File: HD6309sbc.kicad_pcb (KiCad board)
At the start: 4 copper layers, 99.8 x 99.8 mm, 86 parts, among them J1 Conn_01x02_Male, J2 Conn_02x30_Odd_Even, J3 Conn_01x02_Male, J4 Conn_01x07_Socket, J5 Conn_01x07_Socket, J6 PD0, J7 PD1, SW1 SW_Push, U1 HD63C09, U12 74HCT138, U16 74HCT541, U19 74HCT30, U2 DS1813, U3 74AHC1G14, U4 74HCT138, U5 GAL16V8, U6 74HCT574, U7 74HCT574, U8 74HCT541

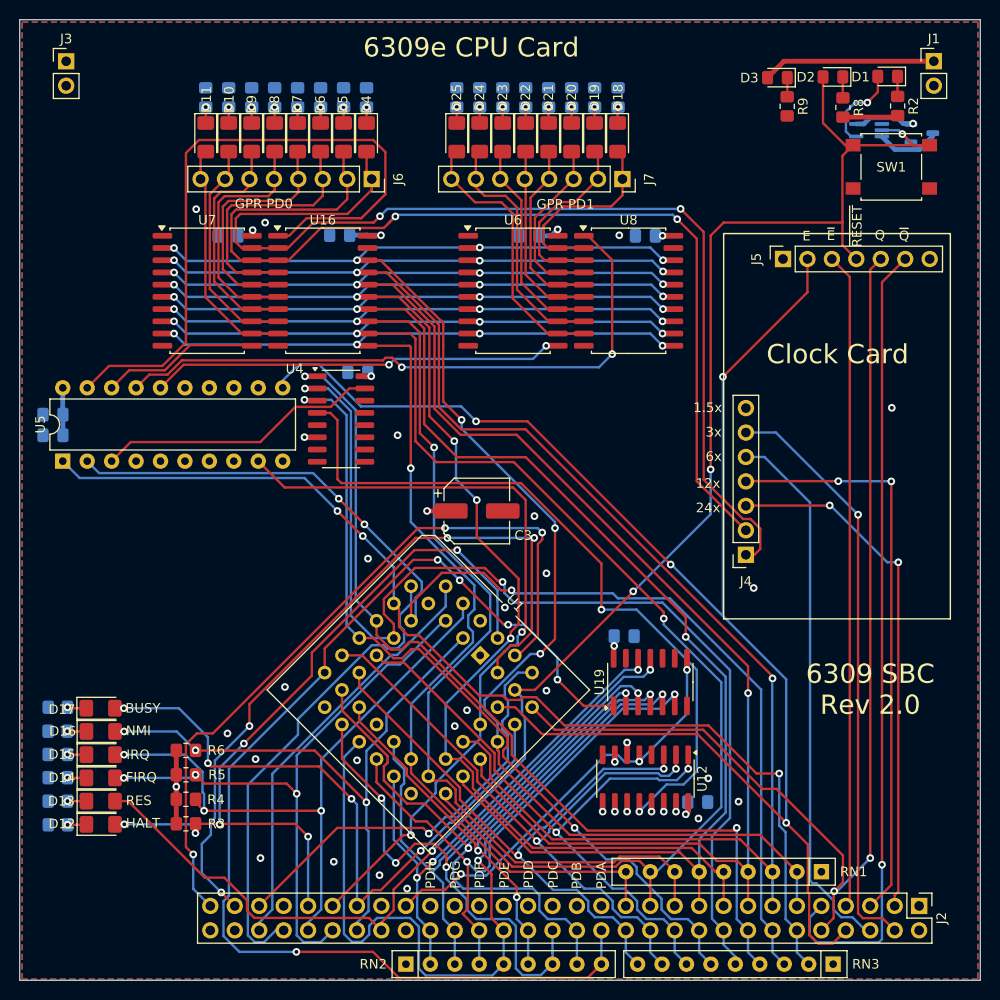
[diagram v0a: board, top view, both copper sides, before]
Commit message: update readme
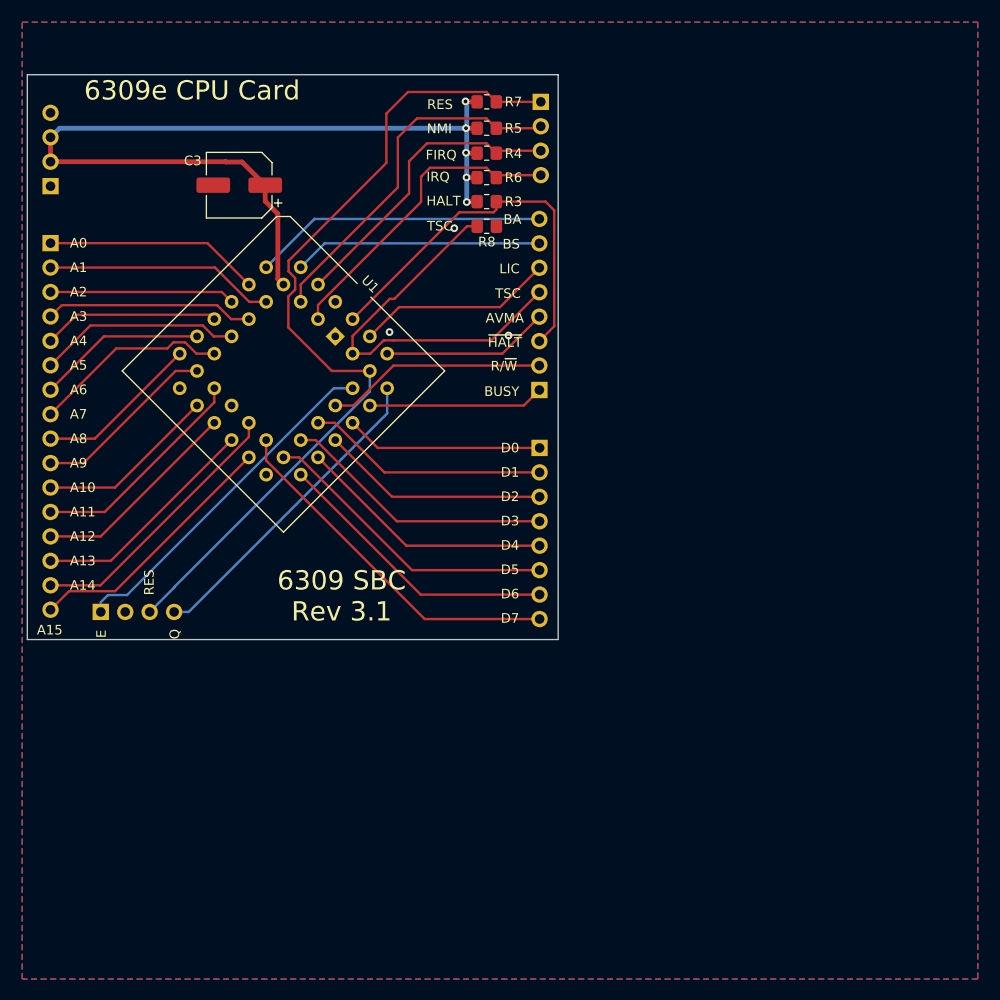
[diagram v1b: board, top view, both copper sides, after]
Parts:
- removed C1, C10, C2, C4, C5, C6, C7, C8, C9: 10uF, Capacitor_SMD:C_0805_2012Metric_Pad1.18x1.45mm_HandSolder
- removed D1: RED, LED_SMD:LED_0805_2012Metric_Pad1.15x1.40mm_HandSolder
- removed D10, D11, D12, D13, D14, D15, D16, D17, D18, D19, D20, D21, D22, D23, D24, D25, D4, D5, D6, D7, D8, D9: LED_Filled, LED_SMD:LED_1206_3216Metric_Pad1.42x1.75mm_HandSolder
- removed D2: YELLOW, LED_SMD:LED_0805_2012Metric_Pad1.15x1.40mm_HandSolder
- removed D3: GREEN, LED_SMD:LED_0805_2012Metric_Pad1.15x1.40mm_HandSolder
- removed J1, J3: Conn_01x02_Male, Connector_PinHeader_2.54mm:PinHeader_1x02_P2.54mm_Vertical
- removed R1, R10, R11, R12, R13, R14, R15, R16, R17, R18, R19, R20, R21, R22, R23, R24, R25, R26, R27, R28, R29: 470R, Resistor_SMD:R_0805_2012Metric_Pad1.20x1.40mm_HandSolder
- removed R2, R9: 330R, Resistor_SMD:R_0805_2012Metric_Pad1.20x1.40mm_HandSolder
- removed RN1, RN2, RN3: 4K7, Resistor_THT:R_Array_SIP9
- removed SW1: SW_Push, Button_Switch_SMD:SW_SPST_B3S-1000
- removed U12, U4: 74HCT138, Package_SO:SOIC-16_3.9x9.9mm_P1.27mm
- removed U16, U8: 74HCT541, Package_SO:SOIC-20W_7.5x12.8mm_P1.27mm
- removed U19: 74HCT30, Package_SO:SOIC-14_3.9x8.7mm_P1.27mm
- removed U2: DS1813, Package_TO_SOT_SMD:SOT-23-3
- removed U3: 74AHC1G14, Package_TO_SOT_SMD:SOT-353_SC-70-5_Handsoldering
- removed U5: GAL16V8, Package_DIP:DIP-20_W7.62mm
- removed U6, U7: 74HCT574, Package_SO:SOIC-20W_7.5x12.8mm_P1.27mm
- added J8: Interrupts, Connector_PinHeader_2.54mm:PinHeader_1x04_P2.54mm_Vertical, B.Cu at (79.6, 33.9)
- J2: value Conn_02x30_Odd_Even -> Address Bus; footprint Connector_PinHeader_2.54mm:PinHeader_2x30_P2.54mm_Vertical -> Connector_PinHeader_2.54mm:PinHeader_1x16_P2.54mm_Vertical; moved to B.Cu
- J4: value Conn_01x07_Socket -> Power; footprint Connector_PinSocket_2.54mm:PinSocket_1x07_P2.54mm_Vertical -> Connector_PinHeader_2.54mm:PinHeader_1x04_P2.54mm_Vertical; moved to B.Cu
- J5: value Conn_01x07_Socket -> quadrature; footprint Connector_PinSocket_2.54mm:PinSocket_1x07_P2.54mm_Vertical -> Connector_PinSocket_2.54mm:PinSocket_1x04_P2.54mm_Vertical; moved to B.Cu
- J6: value PD0 -> Data Bus; footprint Connector_PinSocket_2.54mm:PinSocket_1x08_P2.54mm_Vertical -> Connector_PinHeader_2.54mm:PinHeader_1x08_P2.54mm_Vertical; moved to B.Cu
- J7: value PD1 -> CPU Control; footprint Connector_PinSocket_2.54mm:PinSocket_1x08_P2.54mm_Vertical -> Connector_PinHeader_2.54mm:PinHeader_1x08_P2.54mm_Vertical; moved to B.Cu
- R7: value 470R -> 4.7k; moved to F.Cu
- R8: value 330R -> 4.7k
- moved J2 113.5 mm to (28.6, 48.6), turned to 180 degrees
- moved J4 81.8 mm to (28.6, 42.7), turned to 0 degrees
- moved J5 79.8 mm to (33.8, 86.9), turned to -90 degrees
- moved R5 74.1 mm to (73.9, 36.7)
- moved R4 74.1 mm to (73.9, 39.3)
- moved R3 71.8 mm to (73.9, 44.3)
- moved R6 67.2 mm to (73.9, 41.8)
- moved C3 41.9 mm to (48.2, 42.6), turned to 180 degrees
- moved R8 39.0 mm to (73.9, 46.9), turned to 0 degrees
- moved U1 36.4 mm to (58.2, 58.3)
- moved J6 32.9 mm to (79.4, 69.9), turned to 180 degrees
- moved J7 23.6 mm to (79.4, 63.9), turned to 0 degrees
- moved R7 14.9 mm to (73.9, 33.9), turned to 0 degrees
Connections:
- J2 pad 1: unconnected-(J2-Pin_1-Pad1) -> /A0
- J2 pad 10: Q -> /A9
- J2 pad 11: /D0 -> /A10
- J2 pad 12: /A0 -> /A11
- J2 pad 13: /D1 -> /A12
- J2 pad 14: /A1 -> /A13
- J2 pad 15: /D2 -> /A14
- J2 pad 16: /A2 -> /A15
- J2 pad 2: +5V -> /A1
- J2 pad 3: Clock24 -> /A2
- J2 pad 4: Clock3 -> /A3
- J2 pad 5: Clock12 -> /A4
- J2 pad 6: Clock6 -> /A5
- J2 pad 7: ~{E} -> /A6
- J2 pad 8: E -> /A7
- J2 pad 9: ~{Q} -> /A8
- J4 pad 1: /ClockCard/intD00 -> GND
- J4 pad 2: /ClockCard/intD01 -> +5V
- J4 pad 3: Clock24 -> +5V
- J4 pad 4: Clock12 -> GND
- J5 pad 1: GND -> E
- J5 pad 2: E -> unconnected-(J5-Pin_2-Pad2)
- J5 pad 3: ~{E} -> ~{RESET}
- J5 pad 4: ~{RESET} -> Q
- J6 pad 1: /ClockCard/intD00 -> /D0
- J6 pad 2: /ClockCard/intD01 -> /D1
- J6 pad 3: /ClockCard/intD02 -> /D2
- J6 pad 4: /ClockCard/intD03 -> /D3
- J6 pad 5: /ClockCard/intD04 -> /D4
- J6 pad 6: /ClockCard/intD05 -> /D5
- J6 pad 7: /ClockCard/intD06 -> /D6
- J6 pad 8: /ClockCard/intD07 -> /D7
- J7 pad 1: /intD10 -> BUSY
- J7 pad 2: /intD11 -> R/~{W}
- J7 pad 3: /intD12 -> ~{HALT}
- J7 pad 4: /intD13 -> AVMA
- J7 pad 5: /intD14 -> TSC
- J7 pad 6: /intD15 -> LIC
- J7 pad 7: /intD16 -> BS
- J7 pad 8: /intD17 -> BA
- R7 pad 1: Net-(D5-K) -> +5V
- R7 pad 2: GND -> ~{RESET}
- R8 pad 1: Net-(D2-K) -> TSC
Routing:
- net /D1: track 184.6 -> 25.2 mm, vias 5 -> 0
- net /D2: track 176.6 -> 23.7 mm, vias 5 -> 0
- net /D4: track 171.3 -> 26.8 mm, vias 5 -> 0
- net /D0: track 161.8 -> 20.5 mm, vias 7 -> 0
- net E: track 176.8 -> 36.4 mm, vias 4 -> 0
- net /D6: track 168.1 -> 30.0 mm, vias 5 -> 0
- net /D3: track 154.9 -> 28.3 mm, vias 7 -> 0
- net /D5: track 149.4 -> 31.5 mm, vias 5 -> 0
- net /ClockCard/intD00: track 111.2 -> 0.00 mm, vias 2 -> 0
- net /ClockCard/intD01: track 107.9 -> 0.00 mm, vias 2 -> 0
- net /D7: track 141.8 -> 37.4 mm, vias 5 -> 0
- net /A8: track 120.9 -> 17.1 mm, vias 5 -> 0
- net /A1: track 118.5 -> 23.9 mm, vias 3 -> 0
- net ~{SELPD}: track 91.7 -> 0.00 mm, vias 2 -> 0
- net /A3: track 112.8 -> 21.7 mm, vias 2 -> 0
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- removed copper zone on In2.Cu, net +5V
- removed copper zone on In1.Cu, net GND
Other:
- board size 99.8 x 99.8 mm -> 55.2 x 58.7 mm
- copper layers 4 -> 2
- board text added: "6309 SBC Rev 3.1"
- board text added: "A0"
- board text added: "A1"
- board text added: "A10"
- board text added: "A11"
- board text added: "A12"
- board text added: "A13"
- board text added: "A14"
- board text added: "A15"
- board text added: "A2"
- board text added: "A3"
- board text added: "A4"
- board text added: "A5"
- board text added: "A6"
- board text added: "A7"
- board text added: "A8"
- board text added: "A9"
- board text added: "AVMA"
- board text added: "BA"
- board text added: "BS"
- board text added: "D0"
- board text added: "D1"
- board text added: "D2"
- board text added: "D3"
- board text added: "D4"
- board text added: "D5"
- board text added: "D6"
- board text added: "D7"
- board text added: "LIC"
- board text added: "R/~{W}"
- board text added: "TSC"
- board text added: "~{HALT}"
- board text removed: "1.5x"
- board text removed: "12x"
- board text removed: "24x"
- board text removed: "3x"
- board text removed: "6309 SBC Rev 2.0"
- board text removed: "6x"
- board text removed: "Clock Card"
- board text removed: "GPR PD0"
- board text removed: "GPR PD1"
- board text removed: "PDA"
- board text removed: "PDB"
- board text removed: "PDC"
- board text removed: "PDD"
- board text removed: "PDE"
- board text removed: "PDF"
- board text removed: "PDG"
- board text removed: "PDH"
- board text removed: "~{E}"
- board text removed: "~{Q}"
- board text removed: "~{RESET}"
